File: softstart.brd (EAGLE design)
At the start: 49.2 x 27.3 mm, 9 parts, among them IC1 555

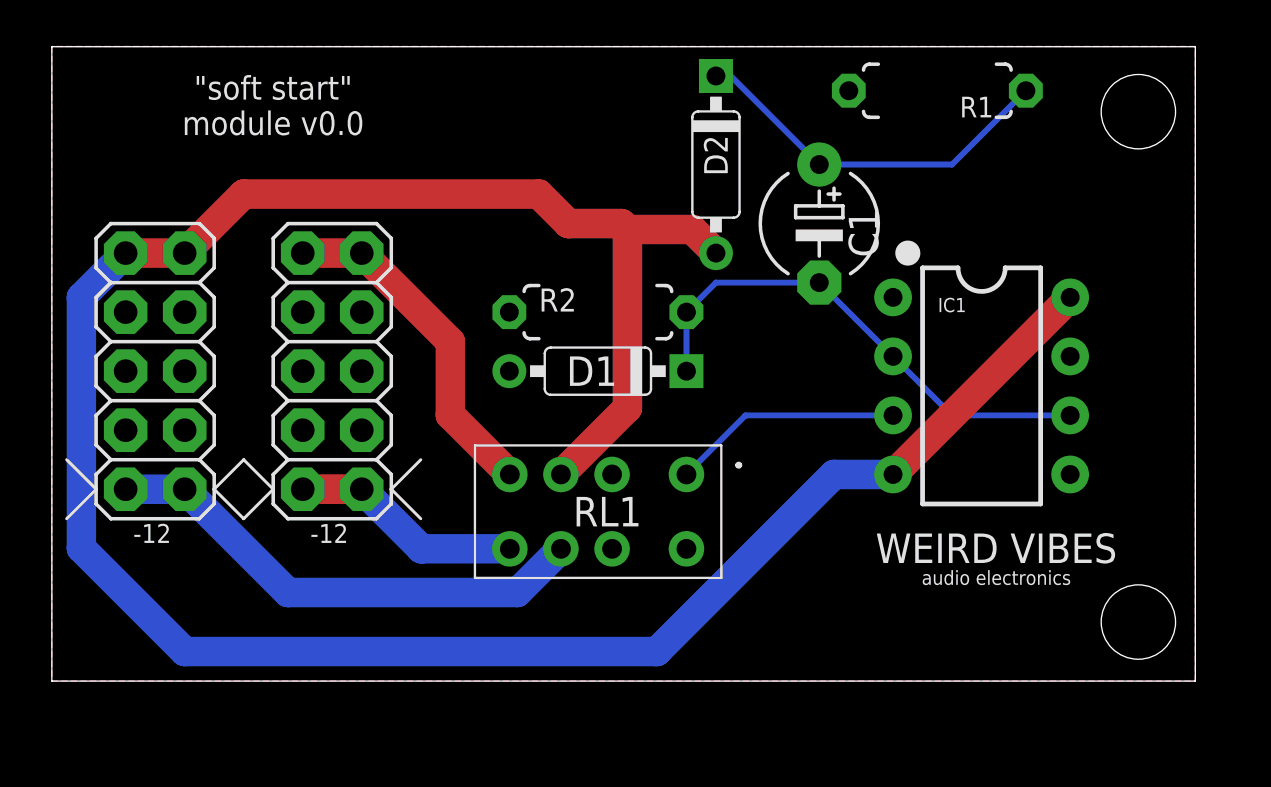
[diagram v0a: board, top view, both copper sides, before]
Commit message: Add files via upload
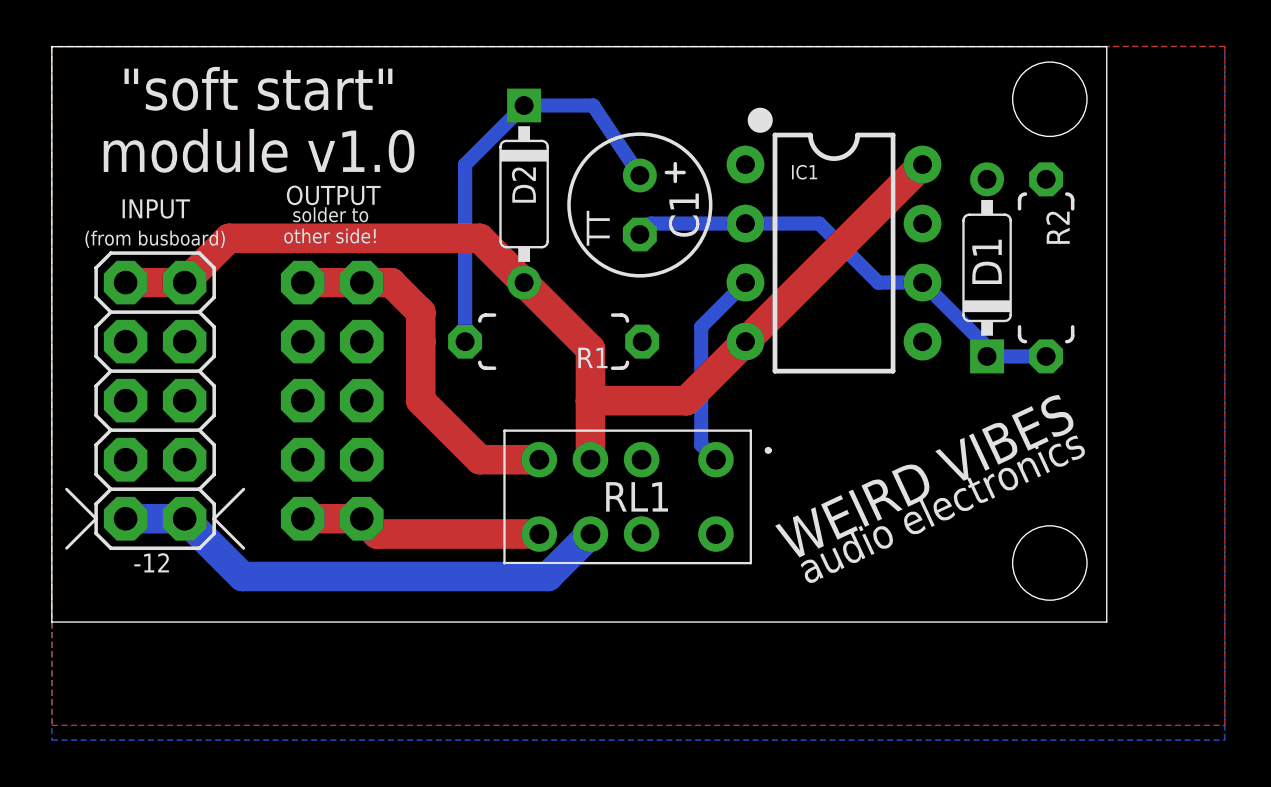
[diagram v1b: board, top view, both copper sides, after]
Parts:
- removed U$1, U$2: RUSS_EURORACK_POWER_SIMPLE10, ES-2144 LPF Module:RUSS_EURORACK_POWER_10
- added POWER_IN, POWER_OUT: RUSS_EURORACK_POWER_SIMPLE10, ES-2144 LPF Module:RUSS_EURORACK_POWER_10
- C1: value (none) -> 47uF; device rcl:E5-5 -> rcl:TT2D6
- D1: value (none) -> 1N4001
- moved R1 19.7 mm to (21.6, 14.6)
- moved R2 19.4 mm to (42.8, 17.8), turned to 270 degrees
- moved D1 17.3 mm to (40.2, 17.8), turned to 90 degrees
- moved IC1 8.54 mm to (33.7, 18.4)
- moved D2 8.35 mm to (20.3, 21.0)
- moved C1 7.76 mm to (25.3, 20.5)
- moved RL1 1.42 mm to (28.6, 9.53)
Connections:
- removed net +12IN: D2.A, IC1.4, IC1.8, RL1.3, U$1.10, U$1.9
- removed net +12SW: RL1.4, U$2.10, U$2.9
- removed net -12IN: RL1.6, U$1.1, U$1.2
- removed net -12SW: RL1.5, U$2.1, U$2.2
- removed net N$2 (its old number): C1.+, D2.C, R1.1
- new net +12_IN: D2.A, IC1.4, IC1.8, POWER_IN.10, POWER_IN.9, RL1.3
- new net +12_SW: POWER_OUT.10, POWER_OUT.9, RL1.4
- new net -12_IN: POWER_IN.1, POWER_IN.2, RL1.6
- new net -12_SW: POWER_OUT.1, POWER_OUT.2, RL1.5
- new net N$1: C1.+, D2.C, R1.2
- net GND: now also POWER_IN.3, POWER_IN.4, POWER_IN.5, POWER_IN.6, POWER_IN.7, POWER_IN.8, POWER_OUT.3, POWER_OUT.4, POWER_OUT.5, POWER_OUT.6, POWER_OUT.7, POWER_OUT.8, R1.1; no longer R1.2, U$1.3, U$1.4, U$1.5, U$1.6, U$1.7, U$1.8, U$2.3, U$2.4, U$2.5, U$2.6, U$2.7, U$2.8
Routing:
- net +12IN: track 103.4 -> 0.00 mm
- net +12_IN: track 0.00 -> 46.0 mm
- net -12_IN: track 0.00 -> 21.8 mm
- net -12IN: track 21.3 -> 0.00 mm
- net N$1: track 0.00 -> 17.8 mm
- net N$2 (its old number): track 16.2 -> 0.00 mm
- net +12_SW: track 0.00 -> 15.6 mm
- net +12SW: track 14.7 -> 0.00 mm
- net -12_SW: track 0.00 -> 10.5 mm
- net -12SW: track 9.97 -> 0.00 mm
- net N$2: track 21.9 -> 20.3 mm
- net N$3: track 9.94 -> 8.67 mm
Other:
- board size 49.2 x 27.3 mm -> 45.4 x 24.8 mm
- board text added: ""soft start" module v1.0"
- board text added: "OUTPUT"
- board text added: "solder to other side!"
- board text removed: ""soft start" module v0.0"
